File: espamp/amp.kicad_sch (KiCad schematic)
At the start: 34 parts, among them U501 TAS5825MRHB

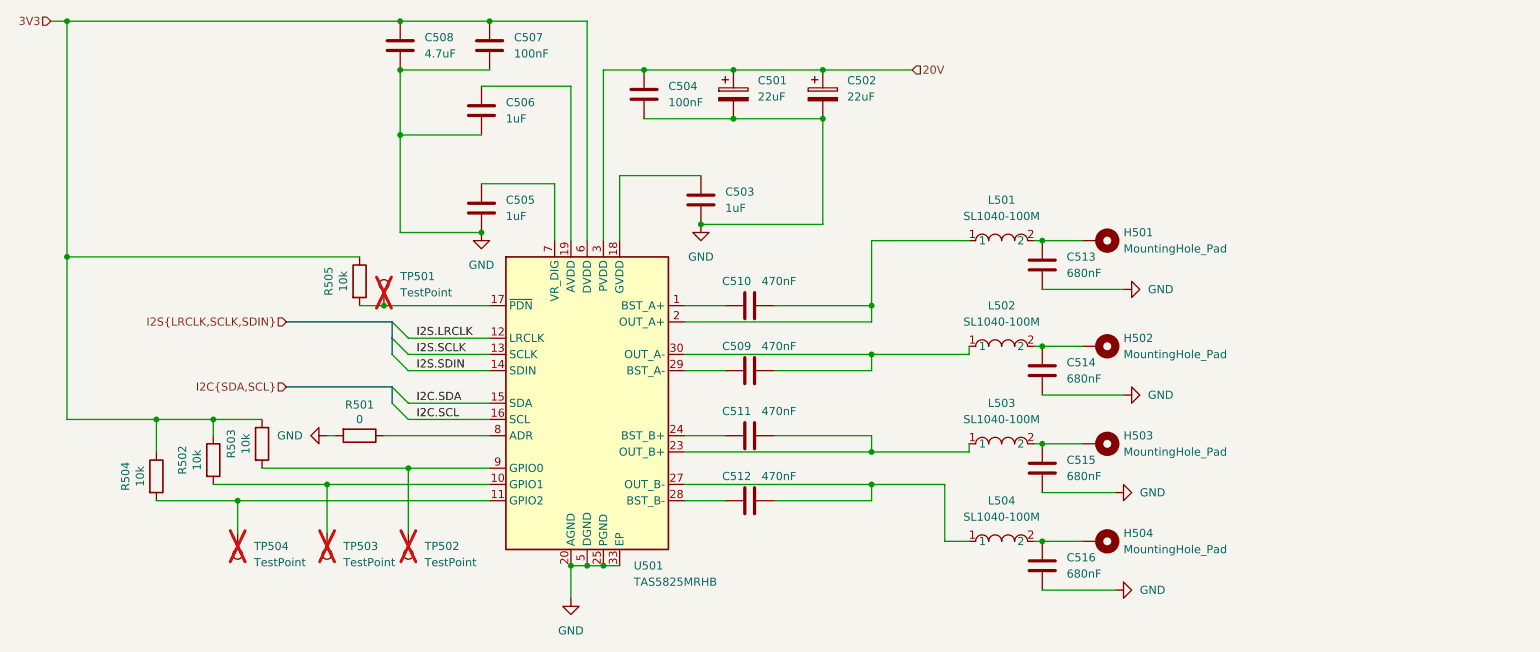
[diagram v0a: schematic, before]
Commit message: first draft of amp layout
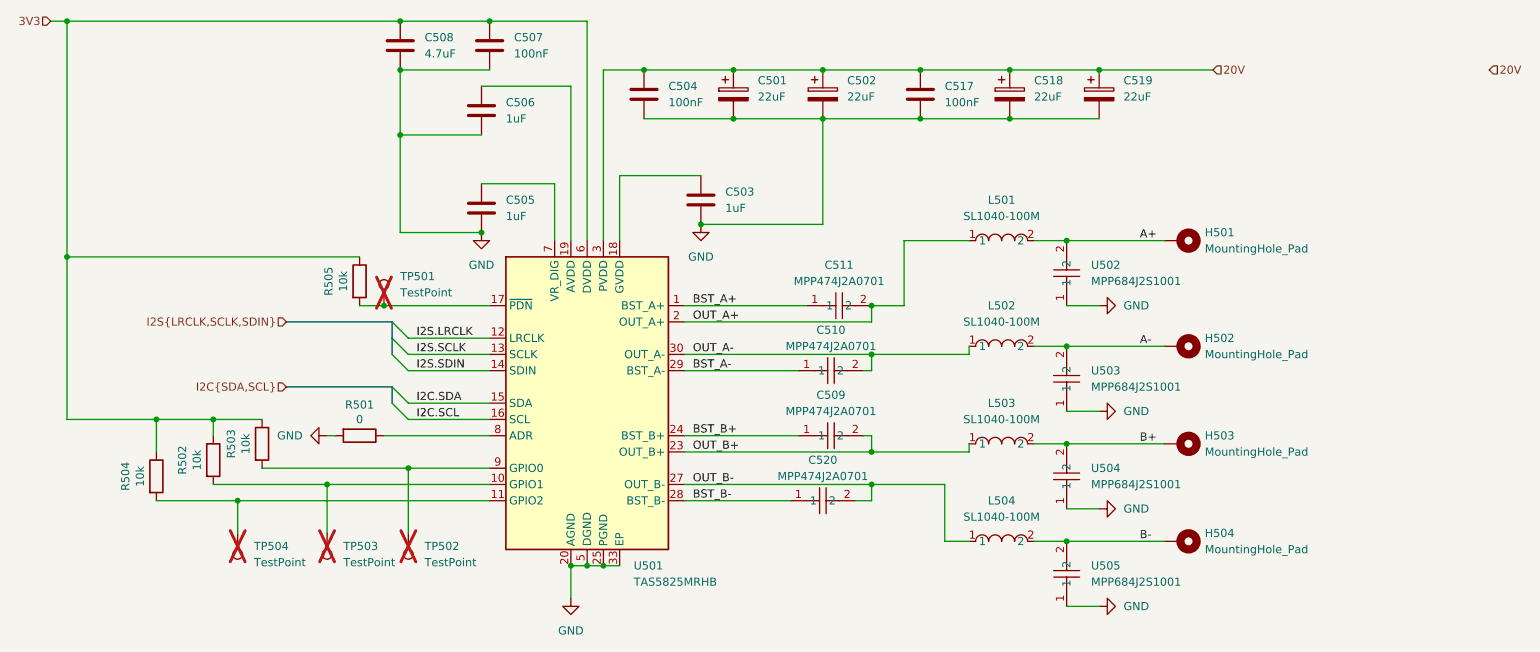
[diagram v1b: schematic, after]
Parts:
- removed C509, C510, C511, C512: 470nF, Capacitor_SMD:C_0603_1608Metric, symbol Device:C
- removed C513, C514, C515, C516: 680nF, Capacitor_SMD:C_0603_1608Metric, symbol Device:C
- added C509, C510, C511, C520: MPP474J2A0701, easyeda2kicad:CAP-TH_L9.5-W3.7-P7.50-D0.5, symbol easyeda2kicad:MPP474J2A0701
- added C517: 100nF, Capacitor_SMD:C_0603_1608Metric, symbol Device:C
- added C518, C519: 22uF, Capacitor_SMD:C_Elec_5x5.8, symbol Device:C_Polarized
- added U502, U503, U504, U505: MPP684J2S1001, easyeda2kicad:CAP-TH_L12.0-W5.8-P10.00-D0.6, symbol easyeda2kicad:MPP684J2S1001
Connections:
- net 20V: now also C517.1, C518.1, C519.1
- net GND: now also C517.2, C518.2, C519.2, U502.1, U503.1, U504.1, U505.1
- net OUT_B-: now reaches L504.1, U501.27 (OUT_B-)
- net OUT_B-: now also C520.2
- net B-: now reaches H504.1, L504.2
- net B-: now also U505.2
- net BST_B+: now reaches U501.24 (BST_B+)
- net BST_B+: now also C509.1
- net OUT_B+: now reaches L503.1, U501.23 (OUT_B+)
- net OUT_B+: now also C509.2
- net A+: now reaches H501.1, L501.2
- net A+: now also U502.2
- net OUT_A-: now reaches L502.1, U501.30 (OUT_A-)
- net OUT_A-: now also C510.2
- net A-: now reaches H502.1, L502.2
- net A-: now also U503.2
- net B+: now reaches H503.1, L503.2
- net B+: now also U504.2
- net BST_A-: now reaches U501.29 (BST_A-)
- net BST_A-: now also C510.1
- net OUT_A+: now reaches L501.1, U501.2 (OUT_A+)
- net OUT_A+: now also C511.2
- net BST_B-: now reaches U501.28 (BST_B-)
- net BST_B-: now also C520.1
- net BST_A+: now reaches U501.1 (BST_A+)
- net BST_A+: now also C511.1
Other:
- moved on the sheet: H501, H502, H503, H504
